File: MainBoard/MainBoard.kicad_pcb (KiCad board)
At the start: 4 copper layers, 35 x 35 mm, 81 parts, among them IC1 MAX30102, IC2 TESEO-LIV3F, J1 PV IN, J2 Conn_Coaxial, J3 Conn_01x30_Female, J4 Conn_Coaxial, J6 Conn_01x04, SW1 SW_DIP_x01, SW2 SW_DIP_x01, SW3 SW_DIP_x01, U1 STM32WB30CEU5A, U2 MAX20361AEWC+, U3 DLF162500LT-5028A1, U4 LSM9DS1, U5 TPS63001, U6 CAT24M01Y, U7 CAT24M01Y, U8 CAT24M01Y, U9 CAT24M01Y, Y1 32 kHz, Y2 Crystal_GND24

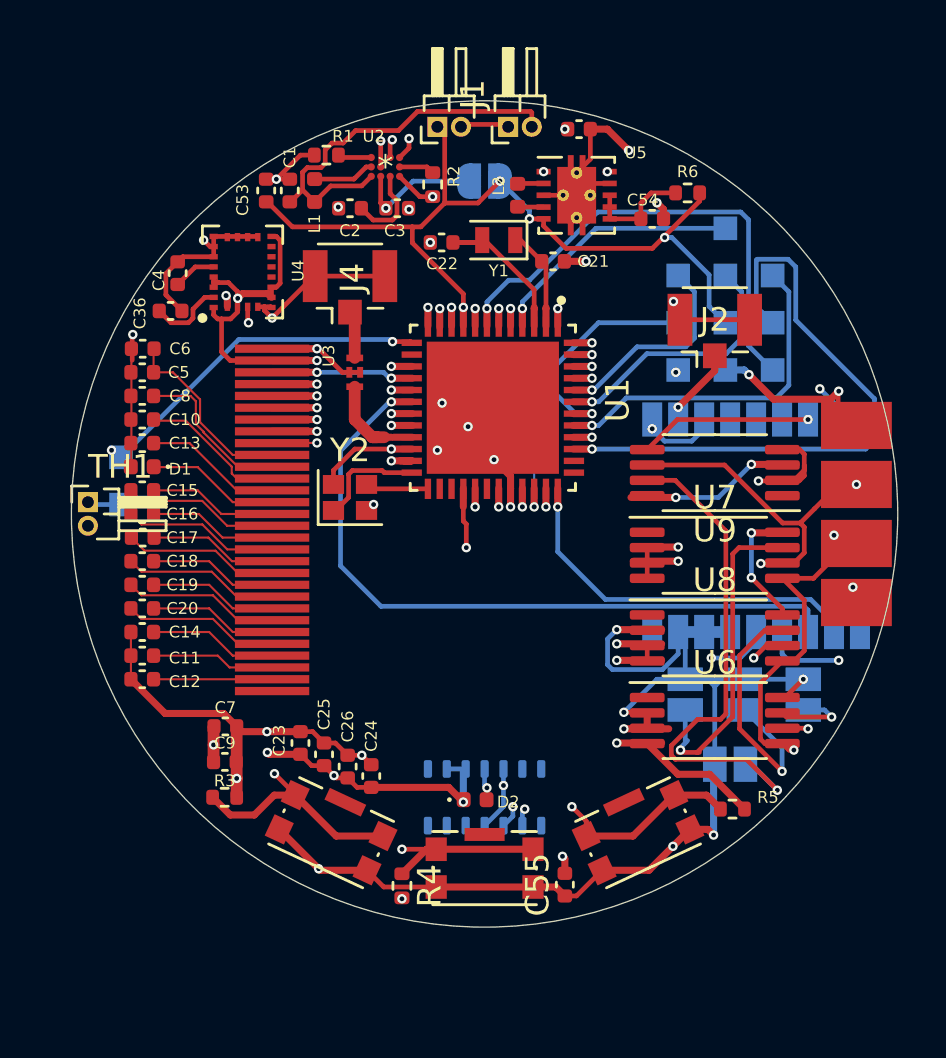
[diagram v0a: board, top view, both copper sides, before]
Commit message: many, many things :)
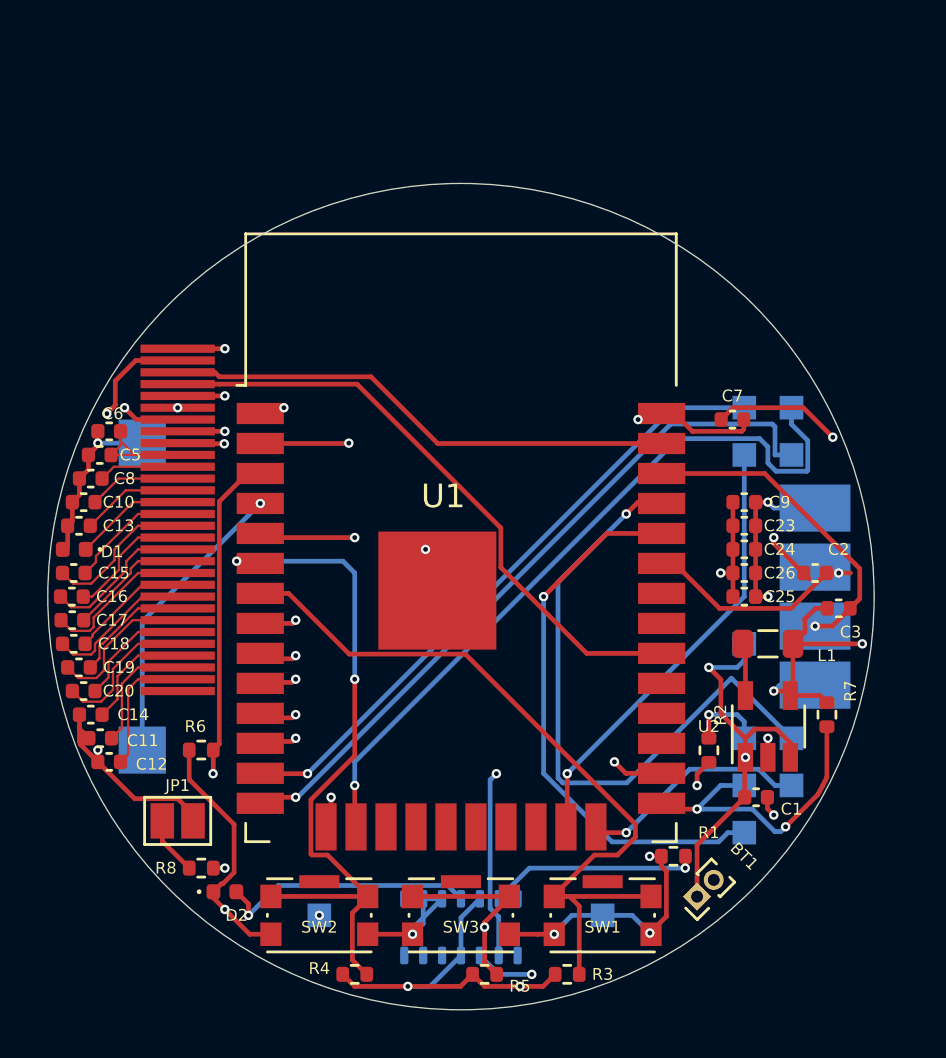
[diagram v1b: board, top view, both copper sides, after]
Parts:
- removed C21, C22: Loading, Capacitor_SMD:C_0402_1005Metric
- removed C36: 100uF, Capacitor_SMD:C_0402_1005Metric
- removed C4: 10nF, Capacitor_SMD:C_0402_1005Metric
- removed C53, C55, C56: 10uF, Capacitor_SMD:C_0402_1005Metric
- removed C54: 0.1uF, Capacitor_SMD:C_0402_1005Metric
- removed IC2: TESEO-LIV3F, libs:SON110P970X1010X230-18N
- removed J1: PV IN, Connector_PinHeader_1.00mm:PinHeader_1x02_P1.00mm_Horizontal
- removed J2, J4: Conn_Coaxial, Connector_Coaxial:U.FL_Hirose_U.FL-R-SMT-1_Vertical
- removed JP2: WP1, Jumper:SolderJumper-2_P1.3mm_Open_Pad1.0x1.5mm
- removed JP3: WP3, Jumper:SolderJumper-2_P1.3mm_Open_Pad1.0x1.5mm
- removed JP4: WP2, Jumper:SolderJumper-2_P1.3mm_Open_Pad1.0x1.5mm
- removed JP5: WP4, Jumper:SolderJumper-2_P1.3mm_Open_Pad1.0x1.5mm
- removed L2: 1uH, Inductor_SMD:L_0402_1005Metric
- removed TH1: Thermistor, Connector_PinHeader_1.00mm:PinHeader_1x02_P1.00mm_Horizontal
- removed U3: DLF162500LT-5028A1, libs:DLF162500LT
- removed U4: LSM9DS1, Package_LGA:LGA-24L_3x3.5mm_P0.43mm
- removed U5: TPS63001, Package_SON:Texas_DRC0010J_ThermalVias
- removed U6, U7, U8, U9: CAT24M01Y, Package_SO:TSSOP-8_4.4x3mm_P0.65mm
- removed Y1: 32 kHz, Crystal:Crystal_SMD_2012-2Pin_2.0x1.2mm
- removed Y2: Crystal_GND24, Crystal:Crystal_SMD_2016-4Pin_2.0x1.6mm
- added BZ1: Buzzer, libs:PB9.11-5v, B.Cu at (120.0, 38.5)
- added R7: 2k, Resistor_SMD:R_0402_1005Metric, F.Cu at (149.0, 43.5)
- added R8: 2k, Resistor_SMD:R_0402_1005Metric, F.Cu at (122.5, 50.0)
- BT1: footprint Connector_PinHeader_1.00mm:PinHeader_1x02_P1.00mm_Horizontal -> Connector_PinHeader_1.00mm:PinHeader_1x02_P1.00mm_Vertical
- C1: value 1uF -> 4.5uF
- C2, C3: value 1uF -> 5.7k
- J6: moved to B.Cu
- JP1: value PV EN -> WP; footprint Jumper:SolderJumper-2_P1.3mm_Open_RoundedPad1.0x1.5mm -> Jumper:SolderJumper-2_P1.3mm_Open_Pad1.0x1.5mm; moved to F.Cu
- L1: value INDUCTOR -> 1uH; footprint Inductor_SMD:L_0402_1005Metric -> Inductor_SMD:L_0805_2012Metric
- R1: value 5K -> 2k
- R2: value R_US -> 2k
- R6: value 100 -> 2k
- TP1: value TestPoint -> RST
- TP2: value JTMS_SWDIO -> IO12
- TP3: value JTCK_SWCLK -> IO14
- TP4: value JTDI -> BOOT0
- TP5: value JTDO -> IO13
- TP6: value NJTRST -> IO15
- TP7: value BOOT0 -> BOOT1
- TP8: value Buzzer -> STX
- TP9: value BuzzerGnd -> SRX
- U1: value STM32WB30CEU5A -> ESP32-WROOM-32; footprint libs:STM32WB30CEU5A -> RF_Module:ESP32-WROOM-32
- U2: value MAX20361AEWC+ -> ADP2108AUJ-3.3; footprint libs:MAX20361AEWC&plus_ -> Package_TO_SOT_SMD:TSOT-23-5
- moved BT1 34.4 mm to (143.5, 51.2), turned to 135 degrees
- moved R1 33.1 mm to (142.5, 49.5)
- moved C1 32.4 mm to (146.0, 47.0), turned to 0 degrees
- moved R6 31.3 mm to (122.5, 45.0), turned to 0 degrees
- moved TP8 30.8 mm to (147.5, 44.5), turned to 0 degrees
- moved JP1 30.1 mm to (121.5, 48.0)
- moved TP9 29.8 mm to (145.5, 48.5), turned to 0 degrees
- moved U2 28.7 mm to (146.5, 44.0), turned to 90 degrees
- moved TP10 27.7 mm to (127.5, 52.0)
- moved L1 27.2 mm to (146.5, 40.5), turned to 0 degrees
- moved R2 26.7 mm to (144.0, 45.0)
- moved C3 25.2 mm to (149.5, 39.0)
- moved C7 25.1 mm to (145.0, 31.0)
- moved C2 25.0 mm to (148.5, 37.5), turned to 0 degrees
- moved C9 24.6 mm to (145.5, 34.5)
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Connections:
- C1 pad 1: Net-(C1-Pad1) -> Net-(BT1-Pad1)
- C2 pad 1: Net-(C2-Pad1) -> +3V3
- C2 pad 2: GND -> SDA
- C3 pad 1: Net-(C3-Pad1) -> +3V3
- C3 pad 2: GND -> SCL
- IC1 pad 1: (no net) -> Net-(IC1-Pad1)
- IC1 pad 13: (no net) -> Net-(IC1-Pad13)
- IC1 pad 14: (no net) -> Net-(IC1-Pad14)
- IC1 pad 5: (no net) -> Net-(IC1-Pad5)
- IC1 pad 6: (no net) -> Net-(IC1-Pad6)
- IC1 pad 7: (no net) -> Net-(IC1-Pad7)
- IC1 pad 8: (no net) -> Net-(IC1-Pad8)
- J3 pad 30: (no net) -> Net-(J3-Pad30)
- JP1 pad 1: Net-(C3-Pad1) -> Net-(JP1-Pad1)
- JP1 pad 2: Net-(BT1-Pad1) -> GND
- L1 pad 1: Net-(C1-Pad1) -> Net-(L1-Pad1)
- L1 pad 2: Net-(L1-Pad2) -> +3V3
- R1 pad 1: GND -> +3V3
- R1 pad 2: Net-(R1-Pad2) -> Net-(IC1-Pad13)
- R6 pad 1: Net-(BT1-Pad1) -> +3V3
- R6 pad 2: Net-(C54-Pad1) -> Net-(R2-Pad1)
- TP1 pad 1: Net-(TP1-Pad1) -> Net-(R2-Pad2)
- TP4 pad 1: Net-(TP4-Pad1) -> Net-(R7-Pad1)
- TP7 pad 1: Net-(TP7-Pad1) -> Net-(R8-Pad2)
- TP9 pad 1: GND -> Net-(TP9-Pad1)
- U1 pad 1: +3V3 -> GND
- U1 pad 10: SPI1-SCK -> Net-(J3-Pad5)
- U1 pad 11: Net-(IC2-Pad4) -> Net-(J3-Pad6)
- U1 pad 12: Net-(IC2-Pad5) -> Net-(J3-Pad7)
- U1 pad 13: Net-(TP8-Pad1) -> Net-(TP3-Pad1)
- U1 pad 14: (no net) -> Net-(TP2-Pad1)
- U1 pad 15: Net-(J3-Pad9) -> GND
- U1 pad 16: SPI1-MOSI -> Net-(TP5-Pad1)
- U1 pad 17: Net-(J3-Pad8) -> Net-(U1-Pad17)
- U1 pad 18: TX -> Net-(U1-Pad18)
- U1 pad 19: Net-(J3-Pad7) -> Net-(U1-Pad19)
- U1 pad 2: Net-(C21-Pad1) -> +3V3
- U1 pad 20: +3V3 -> Net-(U1-Pad20)
- U1 pad 22: GND -> Net-(U1-Pad22)
- U1 pad 23: +3V3 -> Net-(TP6-Pad1)
- U1 pad 24: Net-(U1-Pad24) -> Net-(R8-Pad2)
- U1 pad 25: Net-(U1-Pad25) -> Net-(R7-Pad1)
- U1 pad 26: (no net) -> Net-(R5-Pad1)
- U1 pad 27: (no net) -> Net-(U1-Pad27)
- U1 pad 28: Net-(J3-Pad5) -> Net-(U1-Pad28)
- U1 pad 29: Net-(J3-Pad6) -> Net-(U1-Pad29)
- U1 pad 3: Net-(C22-Pad1) -> Net-(R2-Pad1)
- U1 pad 30: (no net) -> SPI1-SCK
- U1 pad 31: +3V3 -> SPI1-MISO
- U1 pad 32: GND -> Net-(U1-Pad32)
- U1 pad 33: +3V3 -> SDA
- U1 pad 34: +3V3 -> Net-(TP9-Pad1)
- U1 pad 35: +3V3 -> Net-(TP8-Pad1)
- U1 pad 36: RX -> SCL
- U1 pad 37: (no net) -> SPI1-MOSI
- U1 pad 38: (no net) -> GND
- U1 pad 39: Net-(TP2-Pad1) -> GND
- U1 pad 4: Net-(TP7-Pad1) -> Net-(BZ1-Pad2)
- U1 pad 5: SCL -> Net-(BT1-Pad1)
- U1 pad 6: SDA -> Net-(R4-Pad1)
- U1 pad 7: Net-(TP1-Pad1) -> Net-(R3-Pad1)
- U1 pad 8: +3V3 -> Net-(J3-Pad8)
- U1 pad 9: Net-(BT1-Pad1) -> Net-(J3-Pad9)
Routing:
- net +3V3: track 214.5 -> 79.0 mm, vias 32 -> 12
- net GND: track 105.3 -> 48.5 mm, vias 35 -> 14
- net SCL: track 85.8 -> 38.1 mm, vias 9 -> 2
- net SDA: track 82.1 -> 34.7 mm, vias 7 -> 2
- net Net-(IC2-Pad4): track 33.9 -> 0.00 mm, vias 2 -> 0
- net Net-(R2-Pad1): track 22.2 -> 52.9 mm, vias 1 -> 2
- net Net-(IC2-Pad5): track 30.7 -> 0.00 mm, vias 2 -> 0
- net TX: track 30.2 -> 0.00 mm, vias 1 -> 0
- net Net-(R8-Pad2): track 0.00 -> 27.9 mm, vias 0 -> 2
- net Net-(TP9-Pad1): track 0.00 -> 23.5 mm, vias 0 -> 1
- net Net-(JP5-Pad1): track 22.2 -> 0.00 mm, vias 1 -> 0
- net Net-(TP1-Pad1): track 20.7 -> 0.00 mm, vias 1 -> 0
- net Net-(TP5-Pad1): track 11.2 -> 31.6 mm
- net Net-(J3-Pad7): track 9.22 -> 28.1 mm
- net Net-(C1-Pad1): track 16.8 -> 0.00 mm
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- added copper zone on In2.Cu, net +3V3
- added copper zone on In1.Cu, net GND
- removed copper zone on In2.Cu, net GND
